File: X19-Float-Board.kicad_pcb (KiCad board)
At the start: 2 copper layers, 100 x 100 mm, 38 parts, among them J1 Motor, J2 Conn_01x04_Pin, Q1 NMOS, SW2 SW_Nidec_CAS-120A1, U2 AMS1117-3.3, U3 STM32G431RBT6, U4 TPS54336ADDA

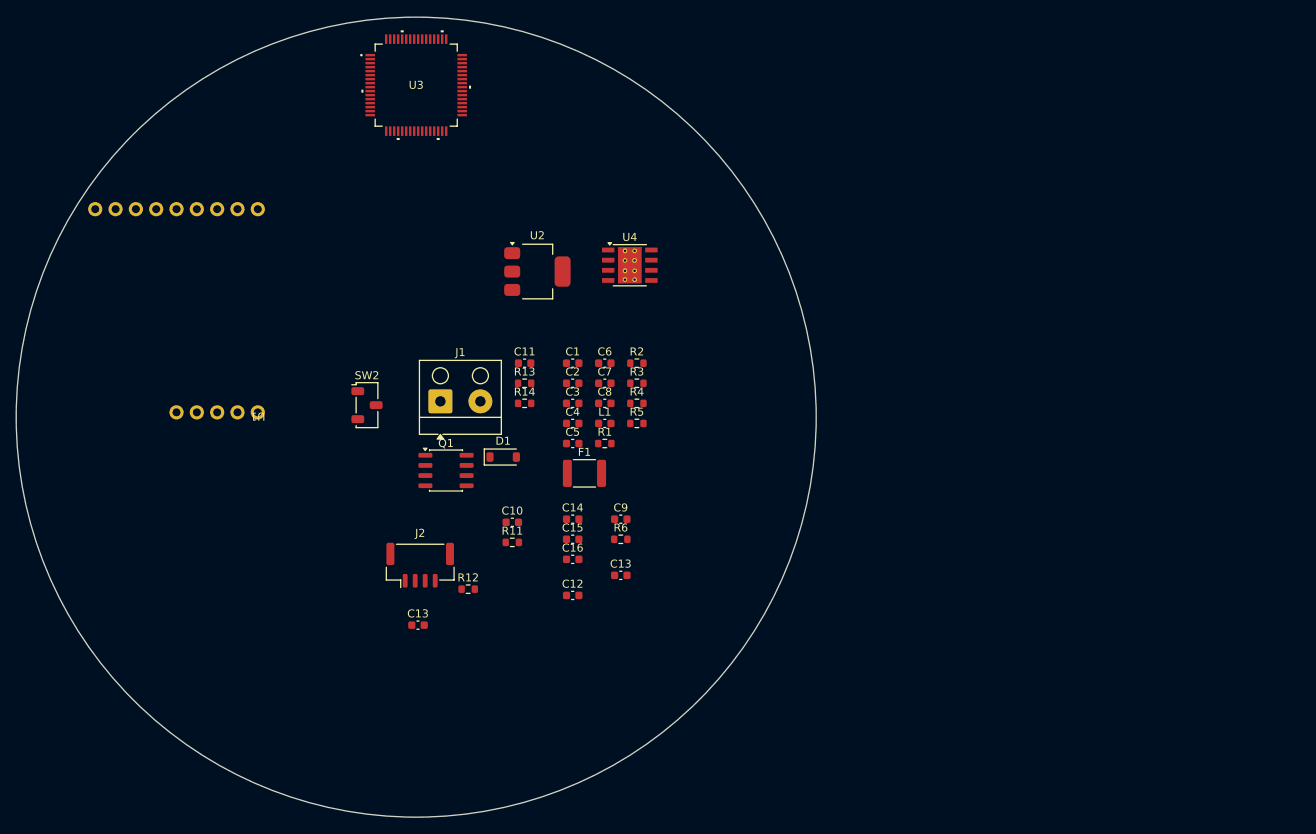
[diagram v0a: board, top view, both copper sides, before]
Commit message: Modifications to power system to support what is required
modified
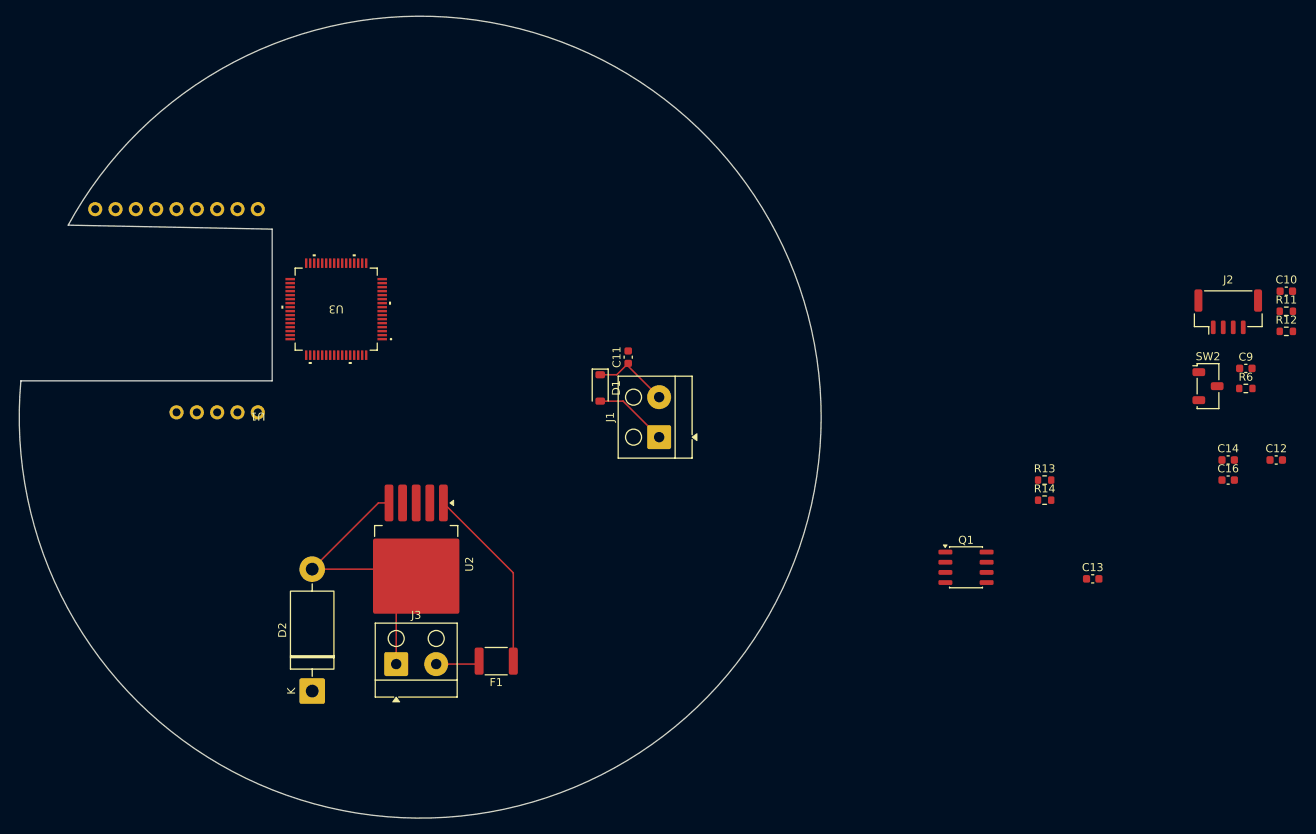
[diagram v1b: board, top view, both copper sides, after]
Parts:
- removed C1: 100nF, Capacitor_SMD:C_0603_1608Metric
- removed the C13 at (150.2, 126.0)
- removed the C13 at (175.6, 119.8)
- removed C15: 4.7µF, Capacitor_SMD:C_0603_1608Metric
- removed C2: 27nF, Capacitor_SMD:C_0603_1608Metric
- removed C3: 10µF, Capacitor_SMD:C_0603_1608Metric
- removed C4: 120pF, Capacitor_SMD:C_0603_1608Metric
- removed C5: .012µF, Capacitor_SMD:C_0603_1608Metric
- removed C6: 0.1µF, Capacitor_SMD:C_0603_1608Metric
- removed C7, C8: 47µF, Capacitor_SMD:C_0603_1608Metric
- removed L1: 15µH, Capacitor_SMD:C_0603_1608Metric
- removed R1: 220kΩ, Resistor_SMD:R_0603_1608Metric
- removed R2: 43.2kΩ, Resistor_SMD:R_0603_1608Metric
- removed R3: 3.74kΩ, Resistor_SMD:R_0603_1608Metric
- removed R4: 100051Ω, Resistor_SMD:R_0603_1608Metric
- removed R5: 19.1kΩ, Resistor_SMD:R_0603_1608Metric
- removed U4: TPS54336ADDA, Package_SO:TI_SO-PowerPAD-8_ThermalVias
- added C13: 100nF, Capacitor_SMD:C_0603_1608Metric, F.Cu at (234.6, 120.2)
- added D2: 1N5822, Diode_THT:D_DO-201AD_P15.24mm_Horizontal, F.Cu at (137.0, 134.2)
- added J3: Screw_Terminal_01x02, TerminalBlock_Altech:Altech_AK100_1x02_P5.00mm, F.Cu at (147.5, 130.9)
- U2: value AMS1117-3.3 -> LM2596S-3.3; footprint Package_TO_SOT_SMD:SOT-223-3_TabPin2 -> Package_TO_SOT_SMD:TO-263-5_TabPin3
- moved R12 107.2 mm to (258.8, 89.3)
- moved J2 105.9 mm to (251.5, 86.8)
- moved SW2 105.2 mm to (249.0, 96.1)
- moved C10 101.0 mm to (258.8, 84.3)
- moved R11 101.0 mm to (258.8, 86.8)
- moved C12 89.6 mm to (257.5, 105.4)
- moved C16 82.5 mm to (251.5, 107.9)
- moved C14 82.3 mm to (251.5, 105.4)
- moved C9 80.4 mm to (253.7, 93.9)
- moved R6 80.4 mm to (253.7, 96.4)
- moved Q1 66.1 mm to (218.7, 118.8)
- moved R13 66.1 mm to (228.6, 107.9)
- moved R14 66.1 mm to (228.6, 110.4)
- moved U2 39.6 mm to (150.0, 118.4), turned to -90 degrees
- moved U3 29.7 mm to (140.0, 86.5), turned to 180 degrees
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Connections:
- U2 pad 1: GND -> 12 V
- U2 pad 2: 3.3 V -> Net-(D2-K)
- U2 pad 3: 5 V -> GND
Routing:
- net GND: track 0.00 -> 38.4 mm
- net 12 V: track 0.00 -> 23.4 mm
- net 12V: track 0.00 -> 9.92 mm
- net Net-(D1-A): track 0.00 -> 9.23 mm
- net Net-(J3-Pin_2): track 0.00 -> 5.51 mm
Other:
- board size 100 x 100 mm -> 100.2 x 100.2 mm
